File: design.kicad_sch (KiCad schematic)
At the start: 20 parts, among them J1 Conn_02x02_Counter_Clockwise, J2 Conn_02x02_Counter_Clockwise, J3 Conn_02x02_Counter_Clockwise, J4 Conn_02x02_Counter_Clockwise, U1 TPS63900

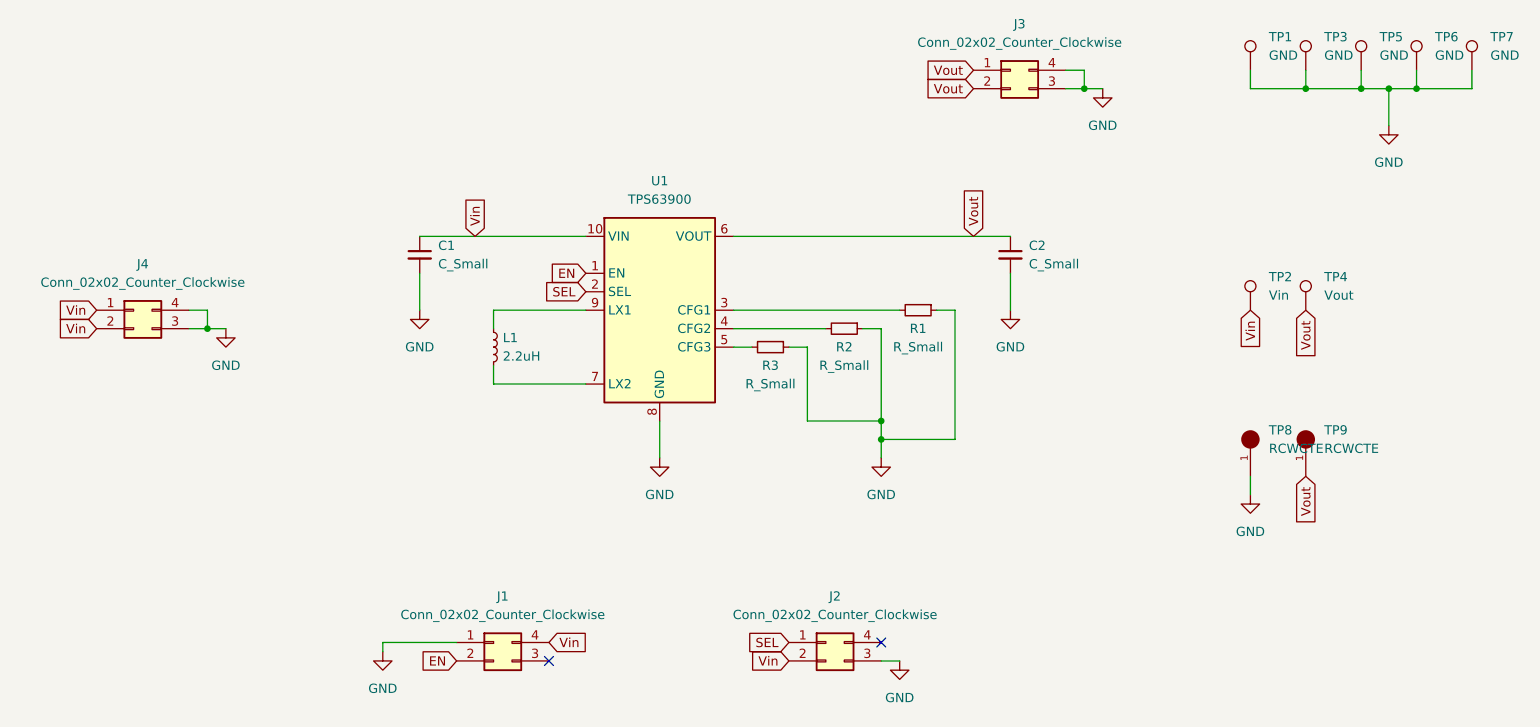
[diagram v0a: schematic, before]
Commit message: update
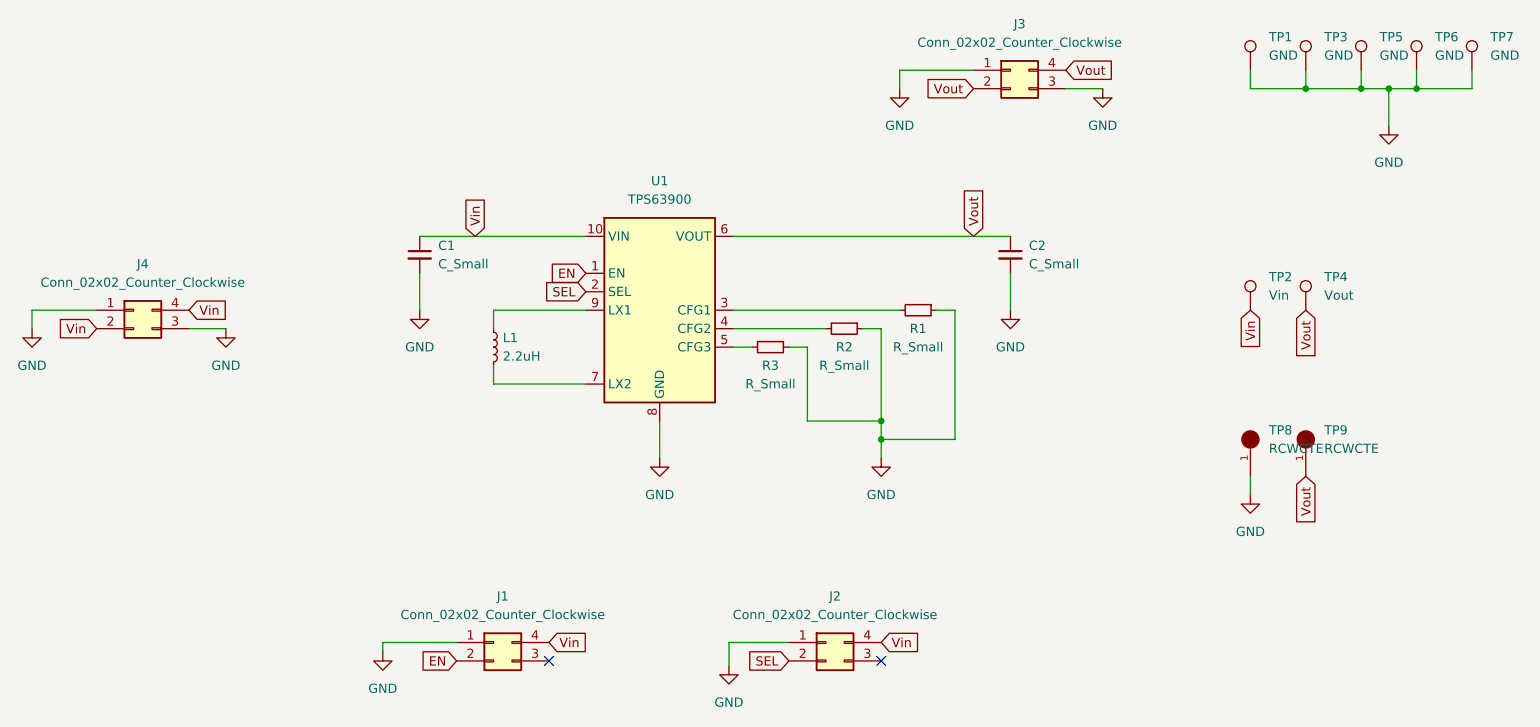
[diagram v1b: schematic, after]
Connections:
- net GND: now also J2.1 (Pin_1), J3.1 (Pin_1), J4.1 (Pin_1); no longer J2.3 (Pin_3), J3.4 (Pin_4), J4.4 (Pin_4)
- net SEL: now also J2.2 (Pin_2); no longer J2.1 (Pin_1)
- net Vin: now also J2.4 (Pin_4), J4.4 (Pin_4); no longer J2.2 (Pin_2), J4.1 (Pin_1)
- net Vout: now also J3.4 (Pin_4); no longer J3.1 (Pin_1)
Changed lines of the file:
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@@
     (comment 4 "<<hash>>")
   )
-  (junction (at 85.09 99.06) (diameter 0) (color 0 0 0 0)
-  )
   (junction (at 247.65 66.04) (diameter 0) (color 0 0 0 0)
   )
@@
   (junction (at 177.8 111.76) (diameter 0) (color 0 0 0 0)
   )
-  (junction (at 205.74 66.04) (diameter 0) (color 0 0 0 0)
-  )
   (junction (at 177.8 114.3) (diameter 0) (color 0 0 0 0)
   )
   (no_connect (at 132.08 144.78))
-  (no_connect (at 177.8 142.24))
+  (no_connect (at 177.8 144.78))
   (wire (pts (xy 251.46 63.5) (xy 251.46 66.04))
     (stroke (width 0) (type default) (color 0 0 0 0))
@@
     (stroke (width 0) (type default) (color 0 0 0 0))
   )
+  (wire (pts (xy 156.845 142.24) (xy 165.1 142.24))
+    (stroke (width 0) (type default) (color 0 0 0 0))
+  )
   (wire (pts (xy 236.22 63.5) (xy 236.22 66.04))
     (stroke (width 0) (type default) (color 0 0 0 0))
@@
     (stroke (width 0) (type default) (color 0 0 0 0))
   )
+  (wire (pts (xy 156.845 145.415) (xy 156.845 142.24))
+    (stroke (width 0) (type default) (color 0 0 0 0))
+  )
   (wire (pts (xy 195.58 91.44) (xy 195.58 96.52))
     (stroke (width 0) (type default) (color 0 0 0 0))
   )
+  (wire (pts (xy 60.96 96.52) (xy 69.85 96.52))
+    (stroke (width 0) (type default) (color 0 0 0 0))
+  )
   (wire (pts (xy 259.08 63.5) (xy 259.08 66.04))
     (stroke (width 0) (type default) (color 0 0 0 0))
   )
+  (wire (pts (xy 180.34 63.5) (xy 190.5 63.5))
+    (stroke (width 0) (type default) (color 0 0 0 0))
+  )
   (wire (pts (xy 157.48 101.6) (xy 160.02 101.6))
     (stroke (width 0) (type default) (color 0 0 0 0))
@@
     (stroke (width 0) (type default) (color 0 0 0 0))
   )
-  (wire (pts (xy 177.8 144.78) (xy 180.34 144.78))
-    (stroke (width 0) (type default) (color 0 0 0 0))
-  )
-  (wire (pts (xy 85.09 96.52) (xy 85.09 99.06))
-    (stroke (width 0) (type default) (color 0 0 0 0))
-  )
   (wire (pts (xy 251.46 66.04) (xy 247.65 66.04))
     (stroke (width 0) (type default) (color 0 0 0 0))
   )
-  (wire (pts (xy 205.74 63.5) (xy 205.74 66.04))
-    (stroke (width 0) (type default) (color 0 0 0 0))
-  )
   (wire (pts (xy 157.48 99.06) (xy 170.18 99.06))
     (stroke (width 0) (type default) (color 0 0 0 0))
   )
-  (wire (pts (xy 203.2 66.04) (xy 205.74 66.04))
-    (stroke (width 0) (type default) (color 0 0 0 0))
-  )
-  (wire (pts (xy 85.09 99.06) (xy 87.63 99.06))
-    (stroke (width 0) (type default) (color 0 0 0 0))
-  )
   (wire (pts (xy 247.65 66.04) (xy 247.65 71.12))
     (stroke (width 0) (type default) (color 0 0 0 0))
@@
     (stroke (width 0) (type default) (color 0 0 0 0))
   )
+  (wire (pts (xy 60.96 99.06) (xy 60.96 96.52))
+    (stroke (width 0) (type default) (color 0 0 0 0))
+  )
   (wire (pts (xy 228.6 63.5) (xy 228.6 66.04))
     (stroke (width 0) (type default) (color 0 0 0 0))
@@
     (stroke (width 0) (type default) (color 0 0 0 0))
   )
-  (wire (pts (xy 82.55 96.52) (xy 85.09 96.52))
-    (stroke (width 0) (type default) (color 0 0 0 0))
-  )
   (wire (pts (xy 167.64 111.76) (xy 177.8 111.76))
     (stroke (width 0) (type default) (color 0 0 0 0))
   )
-  (wire (pts (xy 203.2 63.5) (xy 205.74 63.5))
-    (stroke (width 0) (type default) (color 0 0 0 0))
-  )
-  (wire (pts (xy 82.55 99.06) (xy 85.09 99.06))
+  (wire (pts (xy 82.55 99.06) (xy 87.63 99.06))
     (stroke (width 0) (type default) (color 0 0 0 0))
   )
@@
     (stroke (width 0) (type default) (color 0 0 0 0))
   )
-  (wire (pts (xy 205.74 66.04) (xy 208.28 66.04))
+  (wire (pts (xy 203.2 66.04) (xy 208.28 66.04))
+    (stroke (width 0) (type default) (color 0 0 0 0))
+  )
+  (wire (pts (xy 180.34 66.04) (xy 180.34 63.5))
     (stroke (width 0) (type default) (color 0 0 0 0))
   )
@@
     )
   )
-  (global_label "SEL" (shape input) (at 165.1 142.24 180) (fields_autoplaced)
-    (effects (font (size 1.27 1.27)) (justify right))
-    (property "Referenzen zwischen Schaltplänen" "${INTERSHEET_REFS}" (id 0) (at 159.3891 142.1606 0)
+  (global_label "SEL" (shape input) (at 165.1 144.78 180) (fields_autoplaced)
+    (effects (font (size 1.27 1.27)) (justify right))
+    (property "Referenzen zwischen Schaltplänen" "${INTERSHEET_REFS}" (id 0) (at 159.3891 144.7006 0)
       (effects (font (size 1.27 1.27)) (justify right) hide)
     )
@@
     )
   )
-  (global_label "Vout" (shape input) (at 190.5 63.5 180) (fields_autoplaced)
-    (effects (font (size 1.27 1.27)) (justify right))
-    (property "Referenzen zwischen Schaltplänen" "${INTERSHEET_REFS}" (id 0) (at 184.0634 63.5794 0)
-      (effects (font (size 1.27 1.27)) (justify right) hide)
+  (global_label "Vout" (shape input) (at 203.2 63.5 0) (fields_autoplaced)
+    (effects (font (size 1.27 1.27)) (justify left))
+    (property "Referenzen zwischen Schaltplänen" "${INTERSHEET_REFS}" (id 0) (at 209.6366 63.4206 0)
+      (effects (font (size 1.27 1.27)) (justify left) hide)
     )
   )
@@
     )
   )
-  (global_label "Vin" (shape input) (at 69.85 96.52 180) (fields_autoplaced)
-    (effects (font (size 1.27 1.27)) (justify right))
-    (property "Referenzen zwischen Schaltplänen" "${INTERSHEET_REFS}" (id 0) (at 64.6834 96.4406 0)
-      (effects (font (size 1.27 1.27)) (justify right) hide)
+  (global_label "Vin" (shape input) (at 82.55 96.52 0) (fields_autoplaced)
+    (effects (font (size 1.27 1.27)) (justify left))
+    (property "Referenzen zwischen Schaltplänen" "${INTERSHEET_REFS}" (id 0) (at 87.7166 96.5994 0)
+      (effects (font (size 1.27 1.27)) (justify left) hide)
     )
   )
@@
     )
   )
-  (global_label "Vin" (shape input) (at 165.1 144.78 180) (fields_autoplaced)
-    (effects (font (size 1.27 1.27)) (justify right))
-    (property "Referenzen zwischen Schaltplänen" "${INTERSHEET_REFS}" (id 0) (at 159.9334 144.8594 0)
-      (effects (font (size 1.27 1.27)) (justify right) hide)
+  (global_label "Vin" (shape input) (at 177.8 142.24 0) (fields_autoplaced)
+    (effects (font (size 1.27 1.27)) (justify left))
+    (property "Referenzen zwischen Schaltplänen" "${INTERSHEET_REFS}" (id 0) (at 182.9666 142.1606 0)
+      (effects (font (size 1.27 1.27)) (justify left) hide)
     )
   )
@@
     (pin "1")
   )
-  (symbol (lib_id "power:GND") (at 180.34 144.78 0) (unit 1)
-    (in_bom yes) (on_board yes) (fields_autoplaced)
-    (property "Reference" "#PWR0103" (id 0) (at 180.34 151.13 0)
-      (effects (font (size 1.27 1.27)) hide)
-    )
-    (property "Value" "GND" (id 1) (at 180.34 149.86 0))
-    (property "Footprint" "" (id 2) (at 180.34 144.78 0)
-      (effects (font (size 1.27 1.27)) hide)
-    )
-    (property "Datasheet" "" (id 3) (at 180.34 144.78 0)
+  (symbol (lib_id "power:GND") (at 156.845 145.415 0) (unit 1)
+    (in_bom yes) (on_board yes) (fields_autoplaced)
+    (property "Reference" "#PWR0103" (id 0) (at 156.845 151.765 0)
+      (effects (font (size 1.27 1.27)) hide)
+    )
+    (property "Value" "GND" (id 1) (at 156.845 150.495 0))
+    (property "Footprint" "" (id 2) (at 156.845 145.415 0)
+      (effects (font (size 1.27 1.27)) hide)
+    )
+    (property "Datasheet" "" (id 3) (at 156.845 145.415 0)
       (effects (font (size 1.27 1.27)) hide)
     )
@@
     )
     (property "Datasheet" "" (id 3) (at 147.32 116.84 0)
+      (effects (font (size 1.27 1.27)) hide)
+    )
+    (pin "1")
+  )
+  (symbol (lib_id "power:GND") (at 60.96 99.06 0) (unit 1)
+    (in_bom yes) (on_board yes) (fields_autoplaced)
+    (property "Reference" "#PWR0112" (id 0) (at 60.96 105.41 0)
+      (effects (font (size 1.27 1.27)) hide)
+    )
+    (property "Value" "GND" (id 1) (at 60.96 104.14 0))
+    (property "Footprint" "" (id 2) (at 60.96 99.06 0)
+      (effects (font (size 1.27 1.27)) hide)
+    )
+    (property "Datasheet" "" (id 3) (at 60.96 99.06 0)
       (effects (font (size 1.27 1.27)) hide)
     )
@@
     (pin "1")
   )
+  (symbol (lib_id "power:GND") (at 180.34 66.04 0) (unit 1)
+    (in_bom yes) (on_board yes) (fields_autoplaced)
+    (property "Reference" "#PWR0111" (id 0) (at 180.34 72.39 0)
+      (effects (font (size 1.27 1.27)) hide)
+    )
+    (property "Value" "GND" (id 1) (at 180.34 71.12 0))
+    (property "Footprint" "" (id 2) (at 180.34 66.04 0)
+      (effects (font (size 1.27 1.27)) hide)
+    )
+    (property "Datasheet" "" (id 3) (at 180.34 66.04 0)
+      (effects (font (size 1.27 1.27)) hide)
+    )
+    (pin "1")
+  )
   (symbol (lib_id "Snapeda:RCWCTE") (at 228.6 114.3 90) (unit 1)
     (in_bom yes) (on_board yes) (fields_autoplaced)
@@
       (reference "#PWR0110") (unit 1) (value "GND") (footprint "")
     )
+    (path "/e644cbf8-44e3-4e52-8bfb-67e5d91dff4d"
+      (reference "#PWR0111") (unit 1) (value "GND") (footprint "")
+    )
+    (path "/425ffa30-1c7d-42ae-981f-4a3a2abd9b6c"
+      (reference "#PWR0112") (unit 1) (value "GND") (footprint "")
+    )
     (path "/5597932a-9308-4b20-96c5-01a9581bd15c"
